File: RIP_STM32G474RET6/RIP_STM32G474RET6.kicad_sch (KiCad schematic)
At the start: 35 parts, among them J1 USB_C_Receptacle_USB2.0_14P, J2 Conn_01x04, J3 Conn_01x03, J4 Conn_01x03, J5 Jack-DC, J6 Screw_Terminal_01x02, SW1 SW_Push, SW2 SW_Push, U1 STM32G474RETx, U2 AMS1117-3.3, Y1 8 MHz, Y2 32.768 Mhz

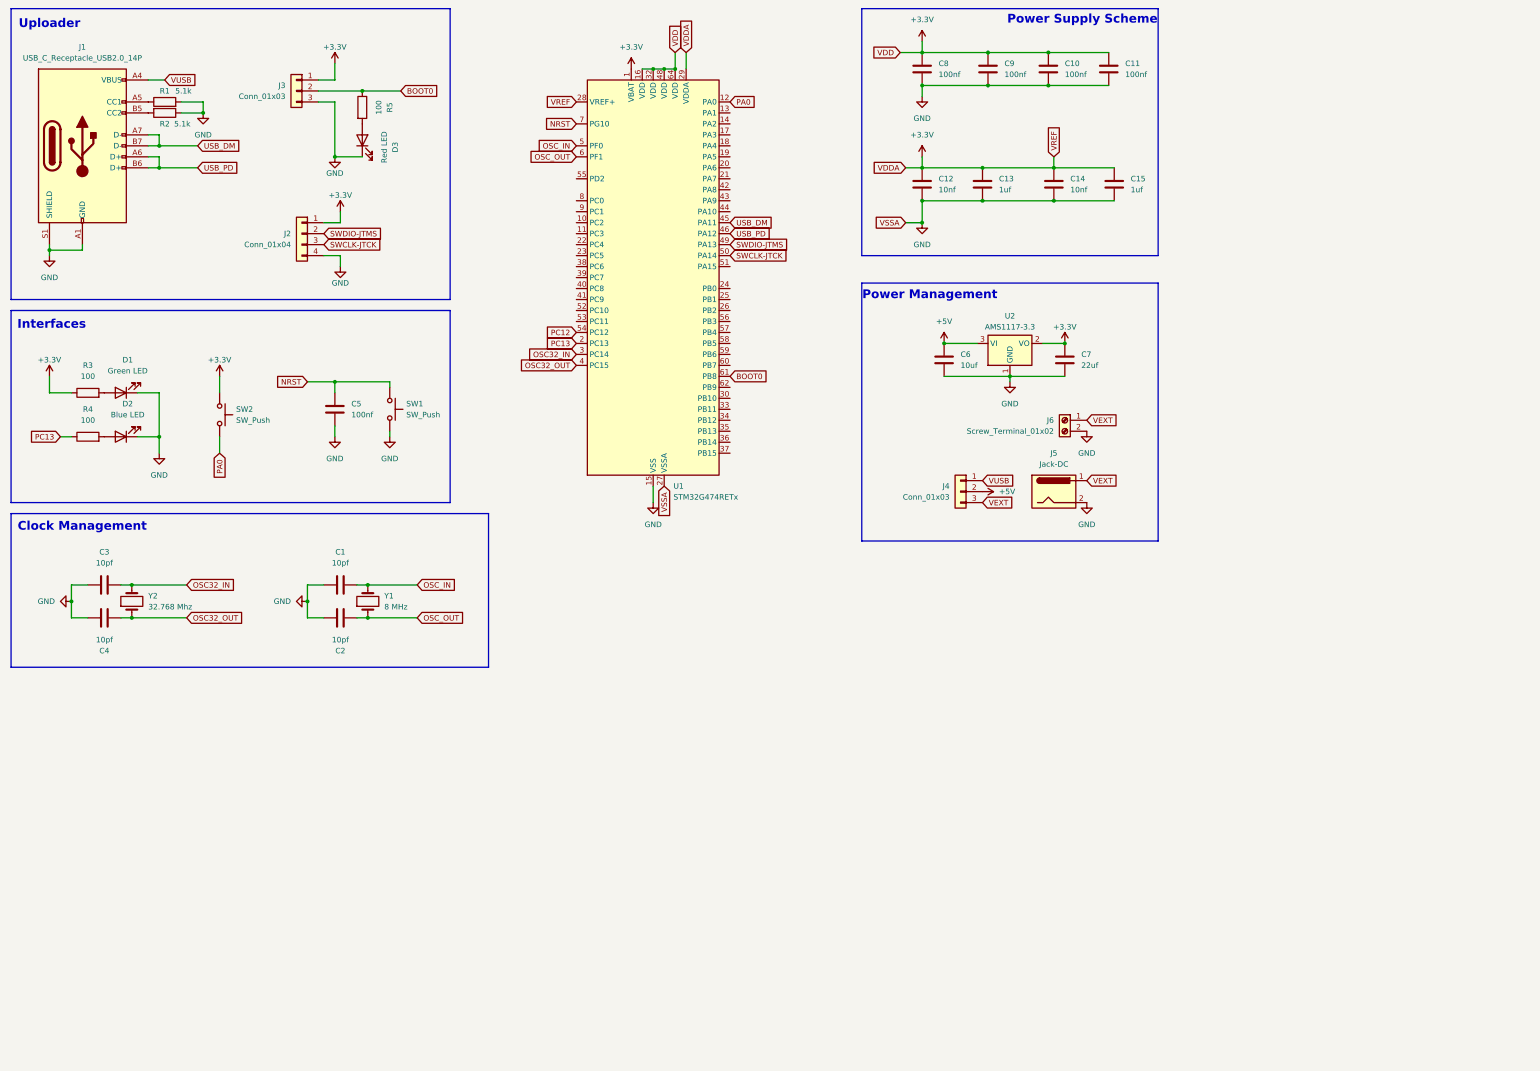
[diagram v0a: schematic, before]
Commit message: rewiring
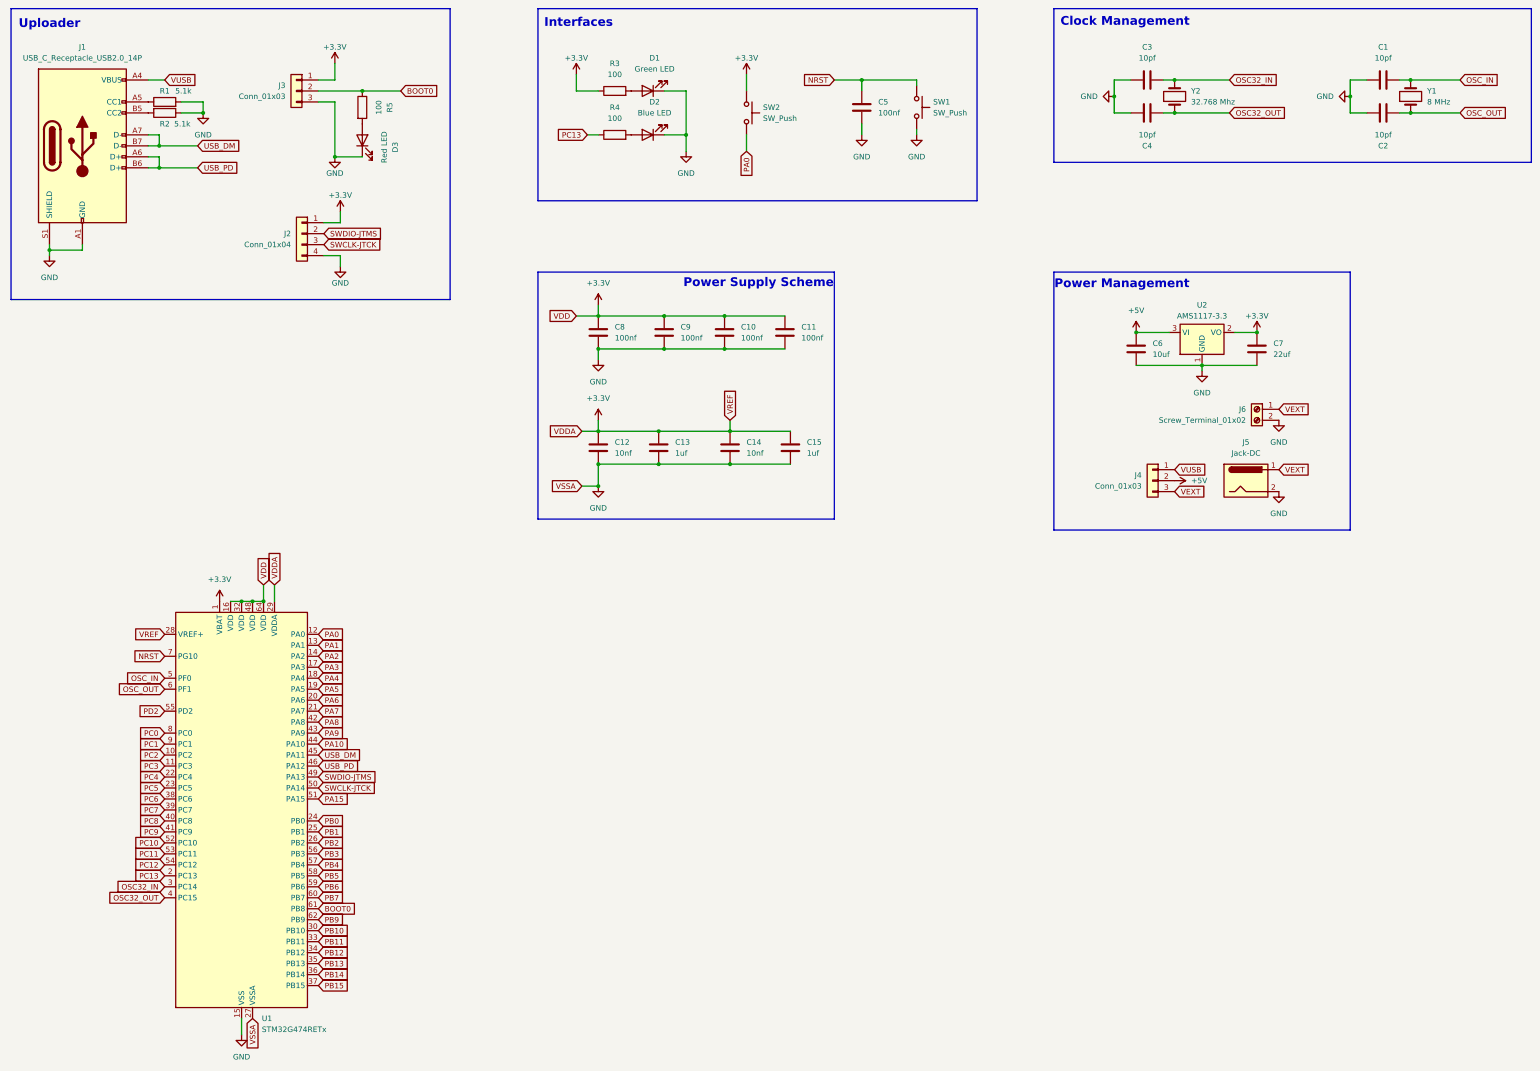
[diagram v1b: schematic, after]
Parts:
- C1, C10, C11, C12, C13, C14, C15, C2, C3, C4, C5, C6, C7, C8, C9: footprint (none) -> Capacitor_SMD:C_0402_1005Metric
- D1, D2, D3: footprint (none) -> LED_SMD:LED_0603_1608Metric
- J1: footprint (none) -> Connector_USB:USB_C_Receptacle_GCT_USB4105-xx-A_16P_TopMnt_Horizontal
- J2: footprint (none) -> Connector_PinHeader_2.54mm:PinHeader_1x04_P2.54mm_Vertical
- J3, J4: footprint (none) -> Connector_PinHeader_2.54mm:PinHeader_1x03_P2.54mm_Vertical
- J5: footprint (none) -> Connector_BarrelJack:BarrelJack_Horizontal
- J6: footprint (none) -> TerminalBlock_Phoenix:TerminalBlock_Phoenix_MKDS-1,5-2-5.08_1x02_P5.08mm_Horizontal
- R1, R2, R3, R4, R5: footprint (none) -> Resistor_SMD:R_0402_1005Metric
- SW1, SW2: footprint (none) -> Button_Switch_SMD:SW_SPST_PTS810
- Y1, Y2: footprint (none) -> Crystal:Crystal_SMD_MicroCrystal_CC7V-T1A-2Pin_3.2x1.5mm
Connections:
- net PC2: now reaches U1.10 (PC2)
- net PC3: now reaches U1.11 (PC3)
- net PA1: now reaches U1.13 (PA1)
- net PA2: now reaches U1.14 (PA2)
- net PA3: now reaches U1.17 (PA3)
- net PA4: now reaches U1.18 (PA4)
- net PA5: now reaches U1.19 (PA5)
- net PA6: now reaches U1.20 (PA6)
- net PA7: now reaches U1.21 (PA7)
- net PC4: now reaches U1.22 (PC4)
- net PC5: now reaches U1.23 (PC5)
- net PB0: now reaches U1.24 (PB0)
- net PB1: now reaches U1.25 (PB1)
- net PB2: now reaches U1.26 (PB2)
- net PB10: now reaches U1.30 (PB10)
- net PB11: now reaches U1.33 (PB11)
- net PB12: now reaches U1.34 (PB12)
- net PB13: now reaches U1.35 (PB13)
- net PB14: now reaches U1.36 (PB14)
- net PB15: now reaches U1.37 (PB15)
- net PC6: now reaches U1.38 (PC6)
- net PC7: now reaches U1.39 (PC7)
- net PC8: now reaches U1.40 (PC8)
- net PC9: now reaches U1.41 (PC9)
- net PA8: now reaches U1.42 (PA8)
- net PA9: now reaches U1.43 (PA9)
- net PA10: now reaches U1.44 (PA10)
- net PA15: now reaches U1.51 (PA15)
- net PC10: now reaches U1.52 (PC10)
- net PC11: now reaches U1.53 (PC11)
- net PD2: now reaches U1.55 (PD2)
- net PB3: now reaches U1.56 (PB3)
- net PB4: now reaches U1.57 (PB4)
- net PB5: now reaches U1.58 (PB5)
- net PB6: now reaches U1.59 (PB6)
- net PB7: now reaches U1.60 (PB7)
- net PB9: now reaches U1.62 (PB9)
- net PC0: now reaches U1.8 (PC0)
- net PC1: now reaches U1.9 (PC1)
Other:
- moved on the sheet: C1, C10, C11, C12, C13, C14, C15, C2, C3, C4, C5, C6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
